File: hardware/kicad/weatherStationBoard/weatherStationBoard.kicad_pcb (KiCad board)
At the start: 2 copper layers, 61 x 31 mm, 28 parts, among them P1 USB_C_Plug_USB2.0, Q1 S8050, Q2 S8050, U1 ESP-12F, U2 CH340G, U4 AMS1117-3.3, Y1 Crystal_GND24_Small

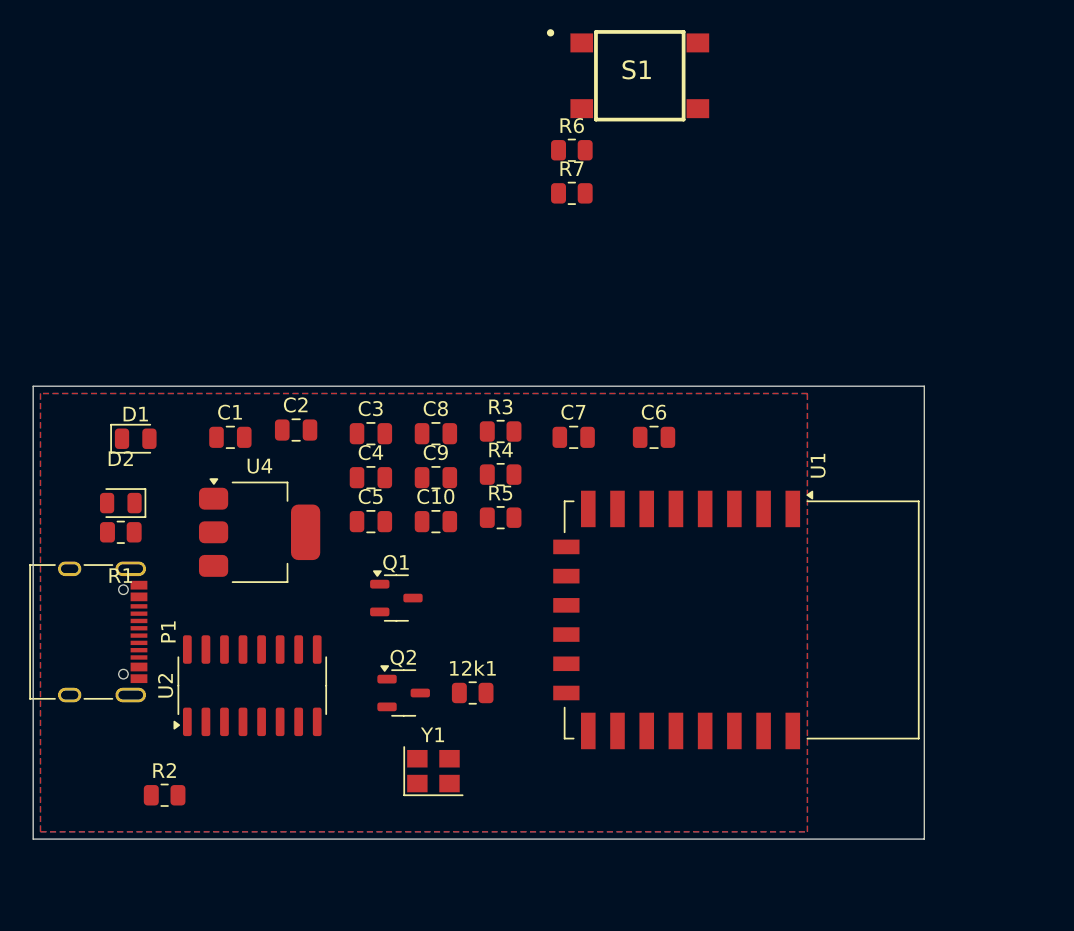
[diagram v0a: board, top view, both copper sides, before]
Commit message: board design prototype no periphery
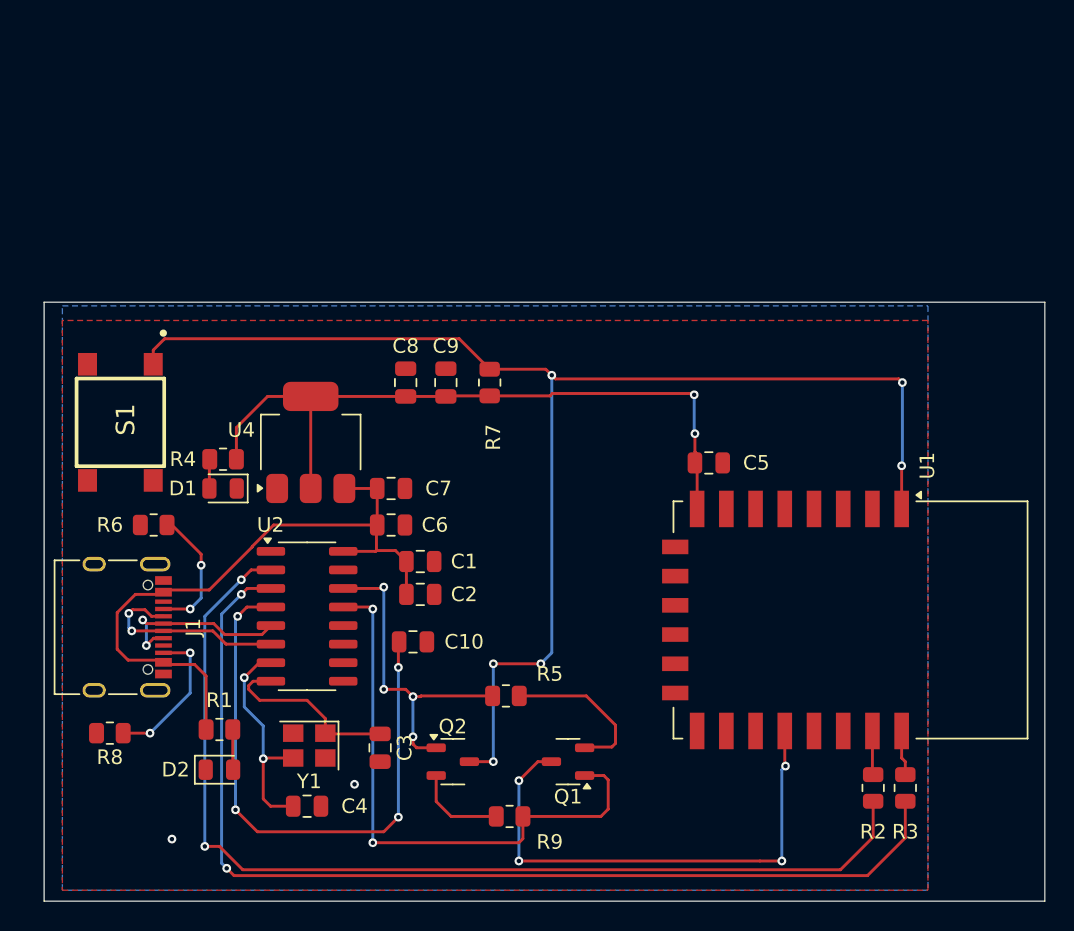
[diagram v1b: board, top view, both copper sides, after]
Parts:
- removed 12k1: R_Small, Resistor_SMD:R_0805_2012Metric
- removed P1: USB_C_Plug_USB2.0, Connector_USB:USB_C_Receptacle_XKB_U262-16XN-4BVC11
- added J1: USB_C_Receptacle_USB2.0_16P, Connector_USB:USB_C_Receptacle_XKB_U262-16XN-4BVC11, F.Cu at (108.2, 61.0)
- added R8: 5k1, Resistor_SMD:R_0805_2012Metric, F.Cu at (108.2, 68.2)
- added R9: 12k, Resistor_SMD:R_0805_2012Metric, F.Cu at (135.6, 74.0)
- moved R2 48.5 mm to (160.5, 72.0), turned to 90 degrees
- moved S1 42.7 mm to (109.0, 47.0), turned to -90 degrees
- moved R6 38.4 mm to (111.2, 54.0), turned to 180 degrees
- moved R3 36.9 mm to (162.7, 72.0), turned to 90 degrees
- moved C5 23.5 mm to (149.2, 49.8)
- moved C4 22.9 mm to (121.8, 73.2)
- moved C3 21.5 mm to (126.8, 69.2), turned to -90 degrees
- moved D2 19.5 mm to (115.8, 70.8), turned to 0 degrees
- moved R4 19.0 mm to (116.0, 49.5), turned to 180 degrees
- moved C6 19.0 mm to (127.5, 54.0)
- moved Q1 16.2 mm to (139.6, 70.2), turned to 180 degrees
- moved C1 15.5 mm to (129.5, 56.5)
- moved R1 15.1 mm to (115.8, 68.0), turned to 0 degrees
- moved R7 14.1 mm to (134.2, 44.2), turned to -90 degrees
- moved C2 14.1 mm to (129.5, 58.8)
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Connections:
- S1 pad 1: unconnected-(S1-Pad1) -> /nRST
- S1 pad 3: unconnected-(S1-Pad3) -> GND
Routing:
- net /nRST: track 0.00 -> 94.1 mm, vias 0 -> 6
- net Net-(U2-RXD): track 0.00 -> 71.9 mm, vias 0 -> 2
- net Net-(U2-TXD): track 0.00 -> 71.4 mm, vias 0 -> 2
- net 3V3: track 0.00 -> 48.8 mm, vias 0 -> 2
- net 5V: track 0.00 -> 46.5 mm
- net Net-(U2-V3): track 0.00 -> 40.1 mm, vias 0 -> 4
- net /DTR: track 0.00 -> 40.0 mm, vias 0 -> 2
- net /GPIO0: track 0.00 -> 35.3 mm, vias 0 -> 4
- net /RTS: track 0.00 -> 22.4 mm, vias 0 -> 4
- net /XI: track 0.00 -> 15.4 mm, vias 0 -> 2
- net Net-(U2-UD-): track 0.00 -> 13.8 mm, vias 0 -> 2
- net Net-(U2-UD+): track 0.00 -> 12.8 mm, vias 0 -> 2
- net /XO: track 0.00 -> 12.8 mm
- net Net-(Q1-B): track 0.00 -> 10.9 mm
- net Net-(J1-CC2): track 0.00 -> 10.3 mm, vias 0 -> 2
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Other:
- board size 61 x 31 mm -> 68.5 x 41 mm
